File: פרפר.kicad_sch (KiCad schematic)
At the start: 41 parts, among them J1 JST_SH_BM03B-SRSS-TB, J2 Hirose_FH12-22S-0.5SH, J5 JST_SH_SM04B-SRSS-TB, J6 JST_SUR_SM02B-SURS-TF, J7 JST_SH_BM03B-SRSS-TB

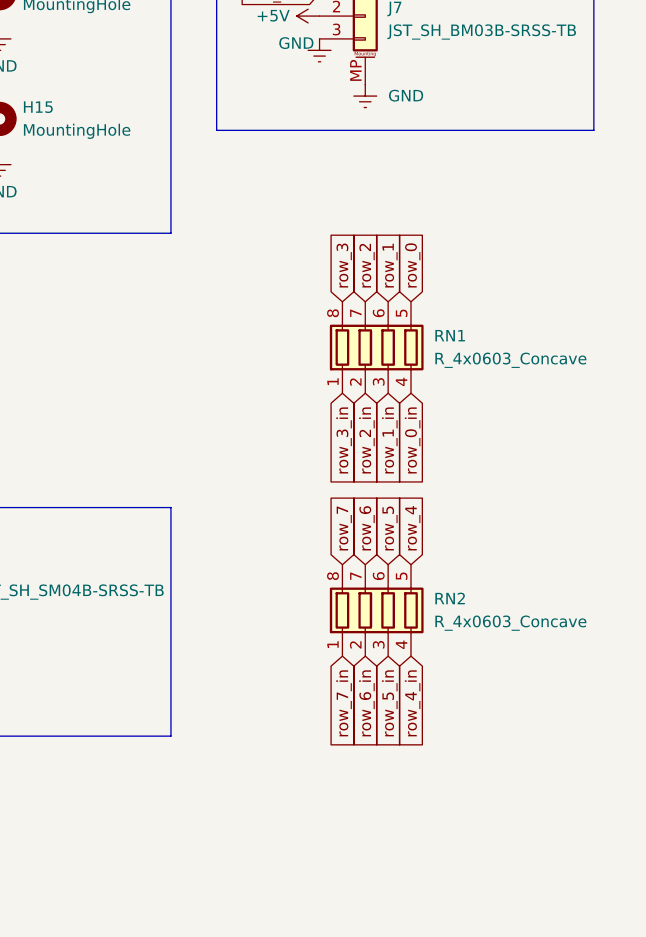
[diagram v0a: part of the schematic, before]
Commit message: coquette parpar mk2 final? try2
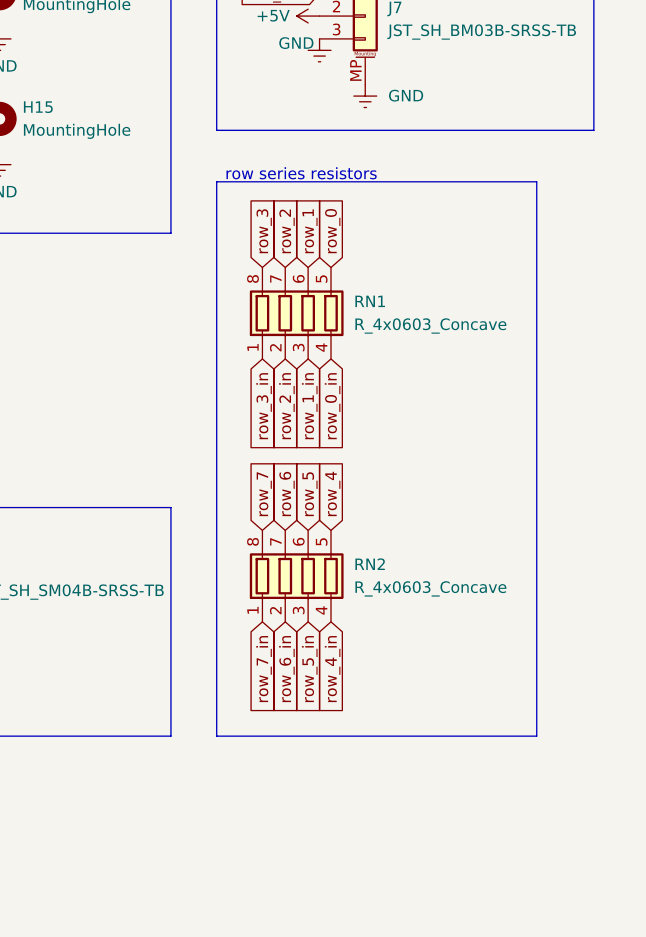
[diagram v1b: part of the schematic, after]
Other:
- note added: "row series resistors"
- moved on the sheet: RN1, RN2
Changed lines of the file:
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@@
 	)
 	(rectangle
+		(start 215.9 98.425)
+		(end 251.46 160.02)
+		(stroke
+			(width 0)
+			(type default)
+		)
+		(fill
+			(type none)
+		)
+	)
+	(rectangle
 		(start 26.67 97.79)
 		(end 71.12 128.27)
@@
 		)
 	)
+	(text "row series resistors"
+		(exclude_from_sim no)
+		(at 225.298 97.79 0)
+		(effects
+			(font
+				(size 1.27 1.27)
+			)
+		)
+	)
 	(text "rgb in"
 		(exclude_from_sim no)
@@
 	(global_label "row_4"
 		(shape input)
-		(at 237.49 140.97 90)
+		(at 228.6 137.16 90)
 		(fields_autoplaced yes)
 		(effects
@@
 		)
 		(property "Intersheetrefs" "${INTERSHEET_REFS}"
-			(at 237.49 133.6103 90)
+			(at 228.6 129.8003 90)
 			(effects
 				(font
@@
 	(global_label "row_5"
 		(shape input)
-		(at 234.95 140.97 90)
+		(at 226.06 137.16 90)
 		(fields_autoplaced yes)
 		(effects
@@
 		)
 		(property "Intersheetrefs" "${INTERSHEET_REFS}"
-			(at 234.95 133.6103 90)
+			(at 226.06 129.8003 90)
 			(effects
 				(font
@@
 	(global_label "row_6"
 		(shape input)
-		(at 232.41 140.97 90)
+		(at 223.52 137.16 90)
 		(fields_autoplaced yes)
 		(effects
@@
 		)
 		(property "Intersheetrefs" "${INTERSHEET_REFS}"
-			(at 232.41 133.6103 90)
+			(at 223.52 129.8003 90)
 			(effects
 				(font
@@
 	(global_label "row_5_in"
 		(shape input)
-		(at 234.95 151.13 270)
+		(at 226.06 147.32 270)
 		(fields_autoplaced yes)
 		(effects
@@
 		)
 		(property "Intersheetrefs" "${INTERSHEET_REFS}"
-			(at 234.95 161.2479 90)
+			(at 226.06 157.4379 90)
 			(effects
 				(font
@@
 	(global_label "row_1_in"
 		(shape input)
-		(at 234.95 121.92 270)
+		(at 226.06 118.11 270)
 		(fields_autoplaced yes)
 		(effects
@@
 		)
 		(property "Intersheetrefs" "${INTERSHEET_REFS}"
-			(at 234.95 132.0379 90)
+			(at 226.06 128.2279 90)
 			(effects
 				(font
@@
 	(global_label "row_0"
 		(shape input)
-		(at 237.49 111.76 90)
+		(at 228.6 107.95 90)
 		(fields_autoplaced yes)
 		(effects
@@
 		)
 		(property "Intersheetrefs" "${INTERSHEET_REFS}"
-			(at 237.49 104.4003 90)
+			(at 228.6 100.5903 90)
 			(effects
 				(font
@@
 	(global_label "row_3_in"
 		(shape input)
-		(at 229.87 121.92 270)
+		(at 220.98 118.11 270)
 		(fields_autoplaced yes)
 		(effects
@@
 		)
 		(property "Intersheetrefs" "${INTERSHEET_REFS}"
-			(at 229.87 132.0379 90)
+			(at 220.98 128.2279 90)
 			(effects
 				(font
@@
 	(global_label "row_1"
 		(shape input)
-		(at 234.95 111.76 90)
+		(at 226.06 107.95 90)
 		(fields_autoplaced yes)
 		(effects
@@
 		)
 		(property "Intersheetrefs" "${INTERSHEET_REFS}"
-			(at 234.95 104.4003 90)
+			(at 226.06 100.5903 90)
 			(effects
 				(font
@@
 	(global_label "row_2_in"
 		(shape input)
-		(at 232.41 121.92 270)
+		(at 223.52 118.11 270)
 		(fields_autoplaced yes)
 		(effects
@@
 		)
 		(property "Intersheetrefs" "${INTERSHEET_REFS}"
-			(at 232.41 132.0379 90)
+			(at 223.52 128.2279 90)
 			(effects
 				(font
@@
 	(global_label "row_0_in"
 		(shape input)
-		(at 237.49 121.92 270)
+		(at 228.6 118.11 270)
 		(fields_autoplaced yes)
 		(effects
@@
 		)
 		(property "Intersheetrefs" "${INTERSHEET_REFS}"
-			(at 237.49 132.0379 90)
+			(at 228.6 128.2279 90)
 			(effects
 				(font
@@
 	(global_label "row_4_in"
 		(shape input)
-		(at 237.49 151.13 270)
+		(at 228.6 147.32 270)
 		(fields_autoplaced yes)
 		(effects
@@
 		)
 		(property "Intersheetrefs" "${INTERSHEET_REFS}"
-			(at 237.49 161.2479 90)
+			(at 228.6 157.4379 90)
 			(effects
 				(font
@@
 	(global_label "row_3"
 		(shape input)
-		(at 229.87 111.76 90)
+		(at 220.98 107.95 90)
 		(fields_autoplaced yes)
 		(effects
@@
 		)
 		(property "Intersheetrefs" "${INTERSHEET_REFS}"
-			(at 229.87 104.4003 90)
+			(at 220.98 100.5903 90)
 			(effects
 				(font
@@
 	(global_label "row_7_in"
 		(shape input)
-		(at 229.87 151.13 270)
+		(at 220.98 147.32 270)
 		(fields_autoplaced yes)
 		(effects
@@
 		)
 		(property "Intersheetrefs" "${INTERSHEET_REFS}"
-			(at 229.87 161.2479 90)
+			(at 220.98 157.4379 90)
 			(effects
 				(font
@@
 	(global_label "row_2"
 		(shape input)
-		(at 232.41 111.76 90)
+		(at 223.52 107.95 90)
 		(fields_autoplaced yes)
 		(effects
@@
 		)
 		(property "Intersheetrefs" "${INTERSHEET_REFS}"
-			(at 232.41 104.4003 90)
+			(at 223.52 100.5903 90)
 			(effects
 				(font
@@
 	(global_label "row_7"
 		(shape input)
-		(at 229.87 140.97 90)
+		(at 220.98 137.16 90)
 		(fields_autoplaced yes)
 		(effects
@@
 		)
 		(property "Intersheetrefs" "${INTERSHEET_REFS}"
-			(at 229.87 133.6103 90)
+			(at 220.98 129.8003 90)
 			(effects
 				(font
@@
 	(global_label "row_6_in"
 		(shape input)
-		(at 232.41 151.13 270)
+		(at 223.52 147.32 270)
 		(fields_autoplaced yes)
 		(effects
@@
 		)
 		(property "Intersheetrefs" "${INTERSHEET_REFS}"
-			(at 232.41 161.2479 90)
+			(at 223.52 157.4379 90)
 			(effects
 				(font
@@
 	(symbol
 		(lib_id "PCM_Resistor_AKL:R_4x0603_Concave")
-		(at 234.95 116.84 0)
+		(at 226.06 113.03 0)
 		(unit 1)
 		(exclude_from_sim no)
@@
 		(fields_autoplaced yes)
 		(property "Reference" "RN1"
-			(at 240.03 115.5699 0)
+			(at 231.14 111.7599 0)
 			(effects
 				(font
@@
 		)
 		(property "Value" "R_4x0603_Concave"
-			(at 240.03 118.1099 0)
+			(at 231.14 114.2999 0)
 			(effects
 				(font
@@
 		)
 		(property "Footprint" "PCM_Resistor_SMD_AKL:R_Array_Concave_4x0603"
-			(at 234.95 129.54 0)
+			(at 226.06 125.73 0)
 			(effects
 				(font
@@
 		)
 		(property "Datasheet" "~"
-			(at 234.95 116.84 0)
+			(at 226.06 113.03 0)
 			(effects
 				(font
@@
 		)
 		(property "Description" "4x0603 SMD Resistor Network, Isolated, European Symbol, Alternate KiCad Library"
-			(at 234.95 116.84 0)
+			(at 226.06 113.03 0)
 			(effects
 				(font
@@
 	(symbol
 		(lib_id "PCM_Resistor_AKL:R_4x0603_Concave")
-		(at 234.95 146.05 0)
+		(at 226.06 142.24 0)
 		(unit 1)
 		(exclude_from_sim no)
@@
 		(fields_autoplaced yes)
 		(property "Reference" "RN2"
-			(at 240.03 144.7799 0)
+			(at 231.14 140.9699 0)
 			(effects
 				(font
@@
 		)
 		(property "Value" "R_4x0603_Concave"
-			(at 240.03 147.3199 0)
+			(at 231.14 143.5099 0)
 			(effects
 				(font
@@
 		)
 		(property "Footprint" "PCM_Resistor_SMD_AKL:R_Array_Concave_4x0603"
-			(at 234.95 158.75 0)
+			(at 226.06 154.94 0)
 			(effects
 				(font
@@
 		)
 		(property "Datasheet" "~"
-			(at 234.95 146.05 0)
+			(at 226.06 142.24 0)
 			(effects
 				(font
@@
 		)
 		(property "Description" "4x0603 SMD Resistor Network, Isolated, European Symbol, Alternate KiCad Library"
-			(at 234.95 146.05 0)
+			(at 226.06 142.24 0)
 			(effects
 				(font
